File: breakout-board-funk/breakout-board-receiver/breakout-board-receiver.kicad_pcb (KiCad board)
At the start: 2 copper layers, 44.2 x 41.2 mm, 5 parts, among them J1 Conn_01x02_Socket, J3 Conn_01x08_Socket, U1 Si4463_eigen

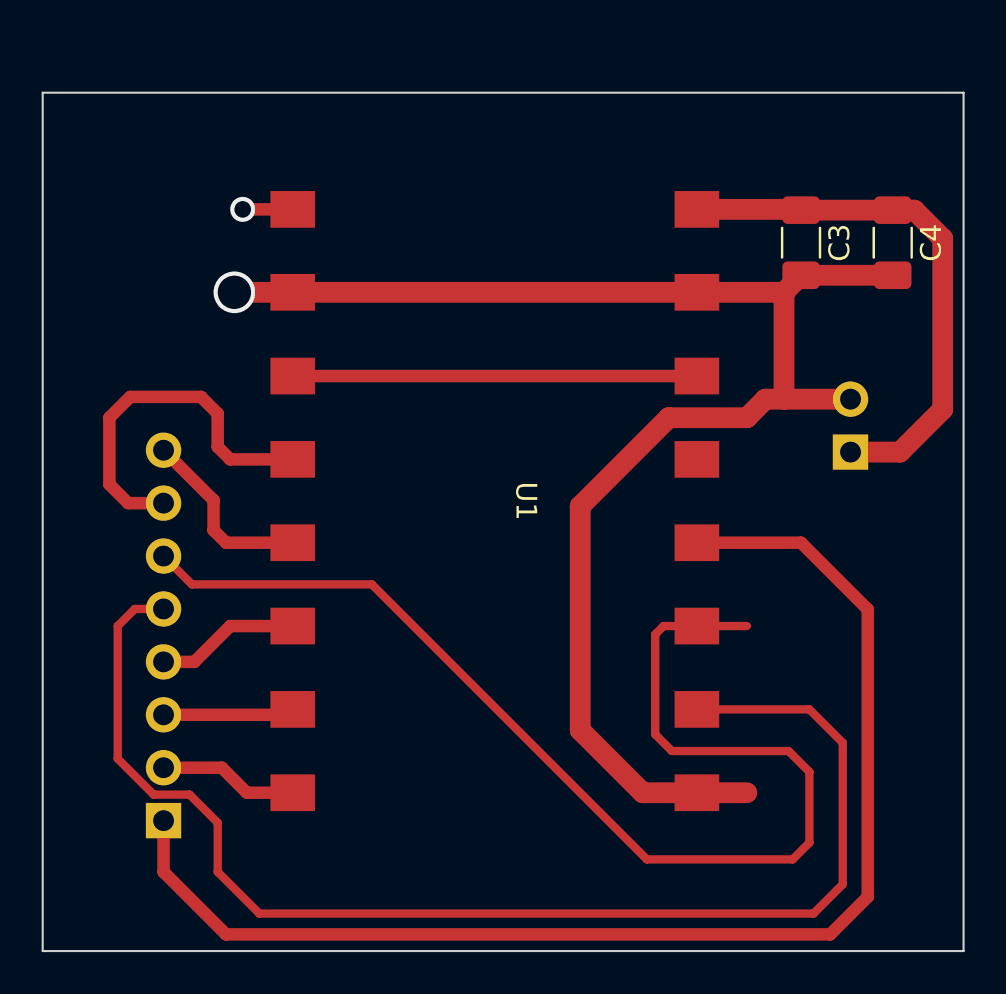
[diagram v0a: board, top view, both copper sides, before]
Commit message: ...
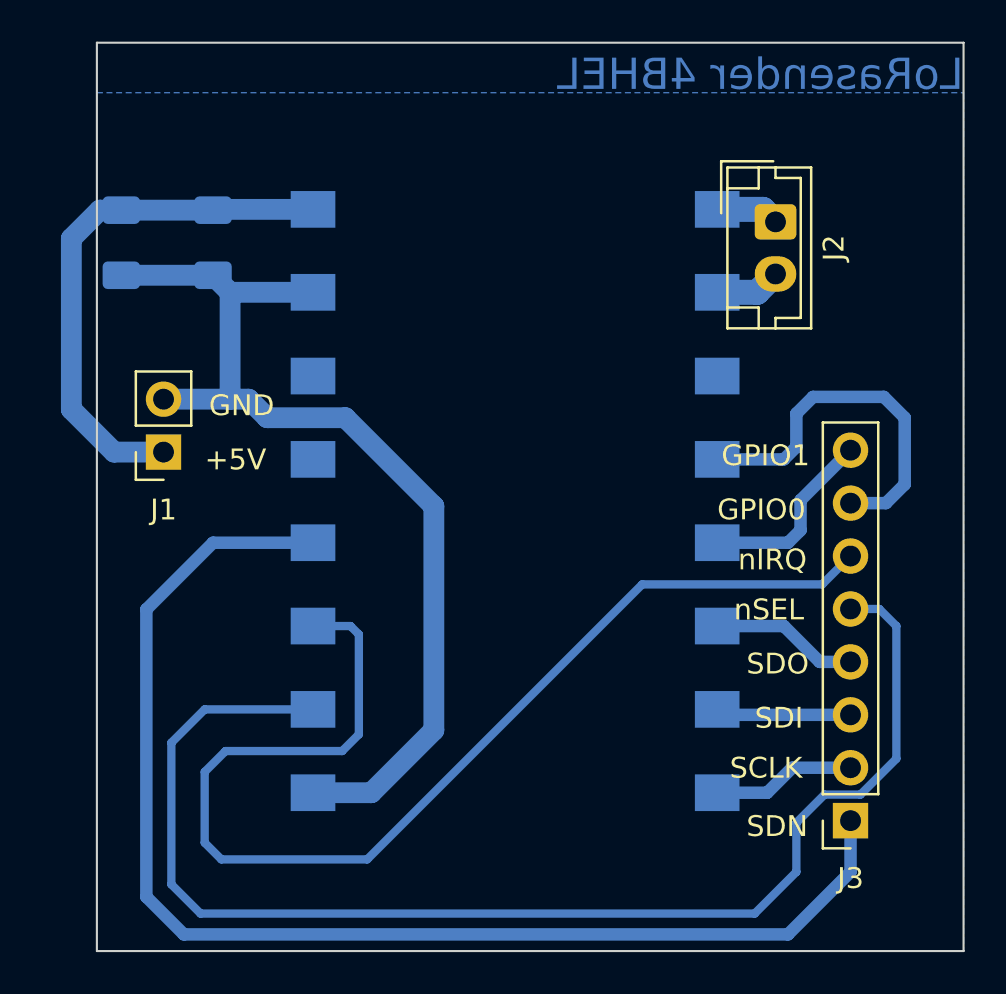
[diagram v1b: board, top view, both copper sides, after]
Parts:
- added J2: Conn_01x02_Socket, Connector_JST:JST_EH_B2B-EH-A_1x02_P2.50mm_Vertical, F.Cu at (187.4, 84.0)
- C3, C4, U1: moved to B.Cu
- J1, J3: moved to F.Cu
- moved C4 37.0 mm to (156.0, 85.0)
- moved J1 33.0 mm to (158.0, 95.0), turned to 180 degrees
- moved J3 33.0 mm to (191.0, 112.7), turned to 180 degrees
- moved C3 28.2 mm to (160.4, 85.0)
- moved U1 0.97 mm to (174.9, 97.4)
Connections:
- U1 pad 10: GND -> /gnd
- U1 pad 11: /NC -> /NC_3
- U1 pad 3: /NC -> /NC_1
- U1 pad 4: /NC -> /NC_2
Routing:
- net GND: track 72.2 -> 47.6 mm, vias 1 -> 0
- net /NC: track 19.4 -> 0.00 mm
- net /gnd: track 0.00 -> 2.96 mm
- net /nIRQ: track 58.3 -> 55.9 mm
- net /Antenne: track 2.40 -> 2.85 mm, vias 1 -> 0
- added copper zone on B.Cu, net (none)
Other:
- board size 44.2 x 41.2 mm -> 41.6 x 43.6 mm
- board text added: "LoRasender 4BHEL"
